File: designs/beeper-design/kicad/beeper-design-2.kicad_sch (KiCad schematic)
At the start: 26 parts, among them U14 EVPBB4A9B000, U15 EVPBB4A9B000, U16 EVPBB4A9B000, U4 DA7212-01UM2, U9 LSM6DSOXTR

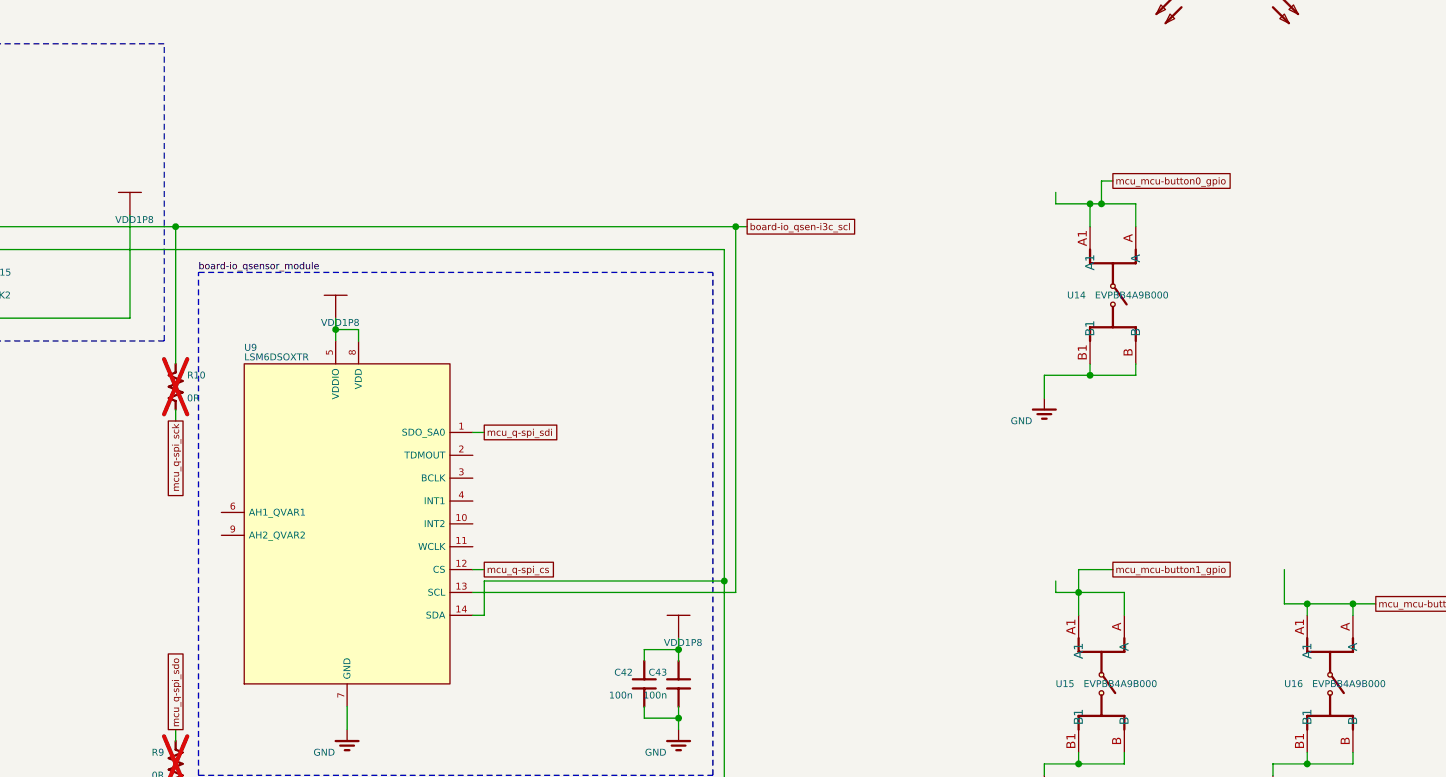
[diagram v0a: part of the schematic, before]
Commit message: updated kicad export
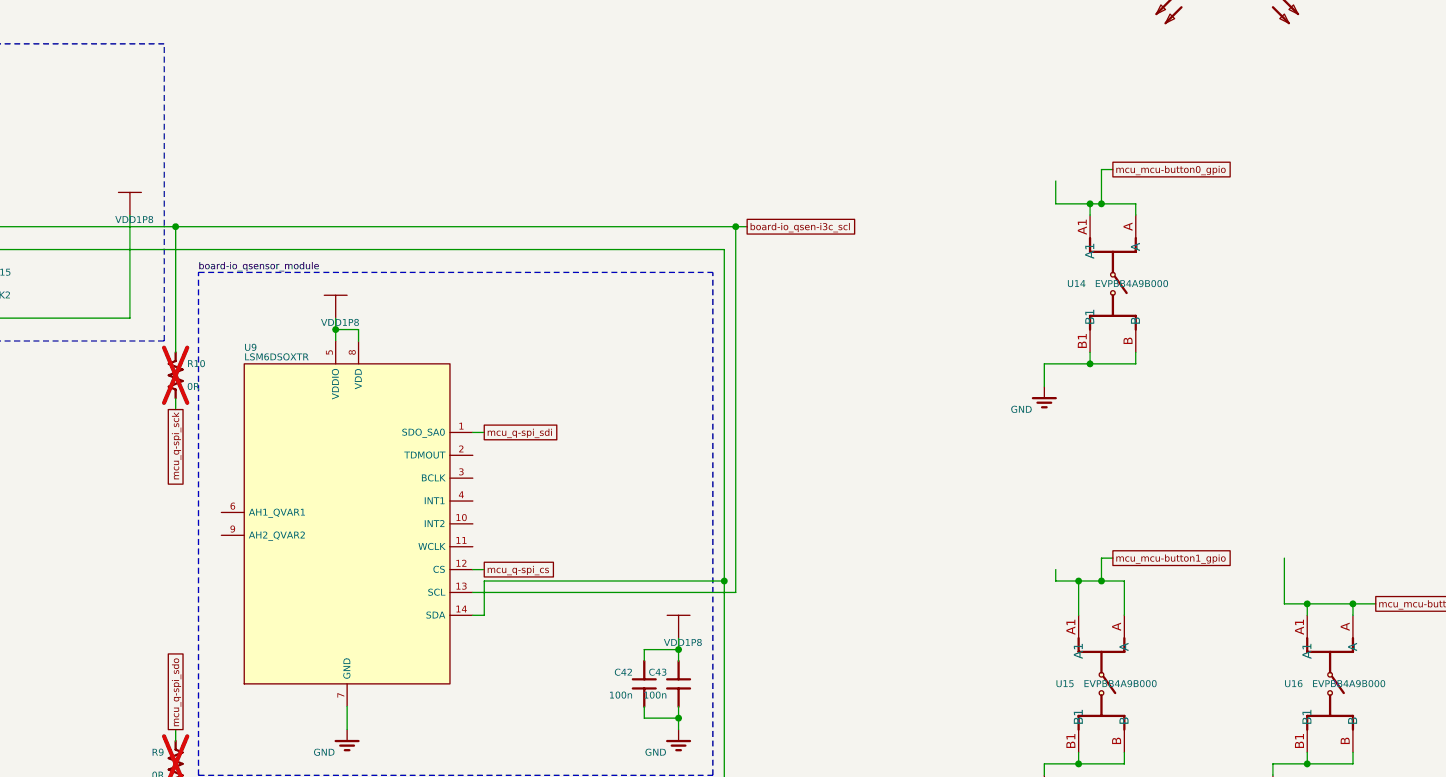
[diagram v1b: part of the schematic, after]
